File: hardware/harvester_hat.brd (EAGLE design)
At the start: 65 x 56.5 mm, 11 parts, among them IC1 7805T, J1 DCJ0202, U1 CAT24C32

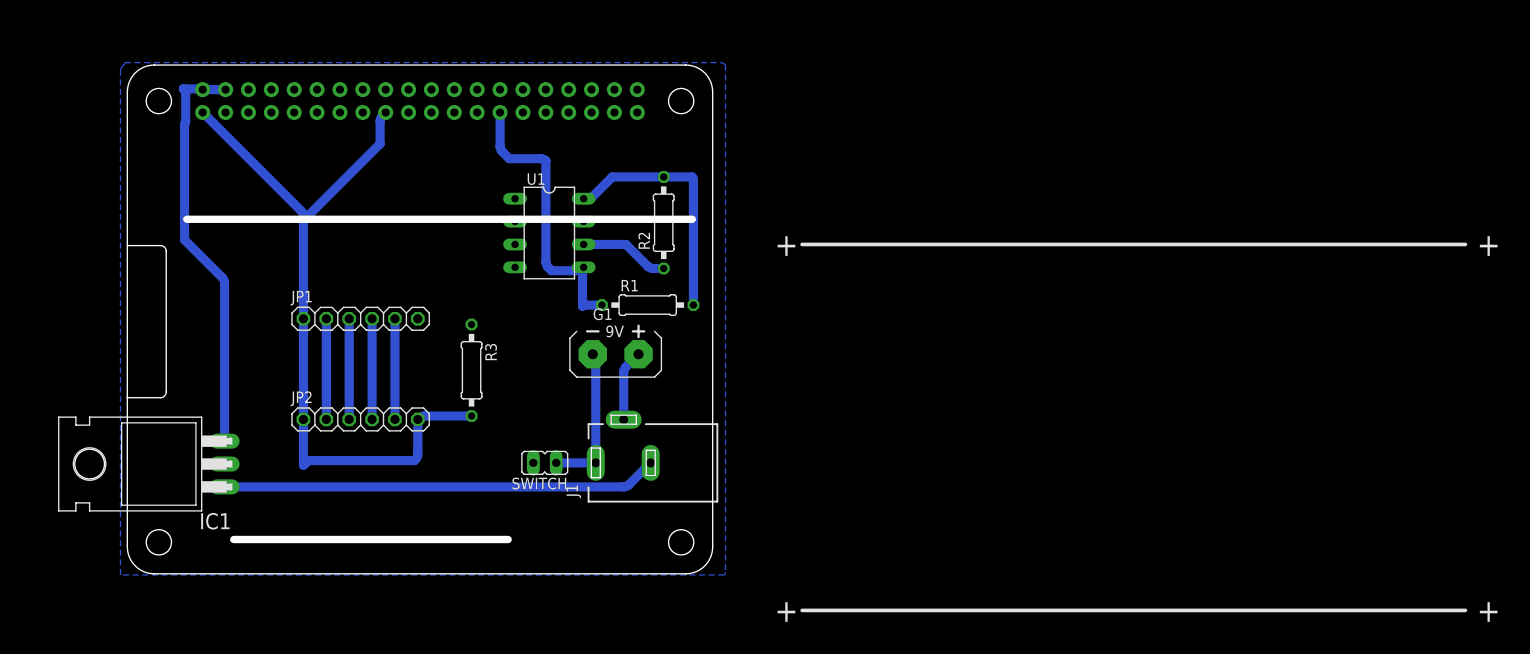
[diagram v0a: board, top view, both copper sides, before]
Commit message: added extra files
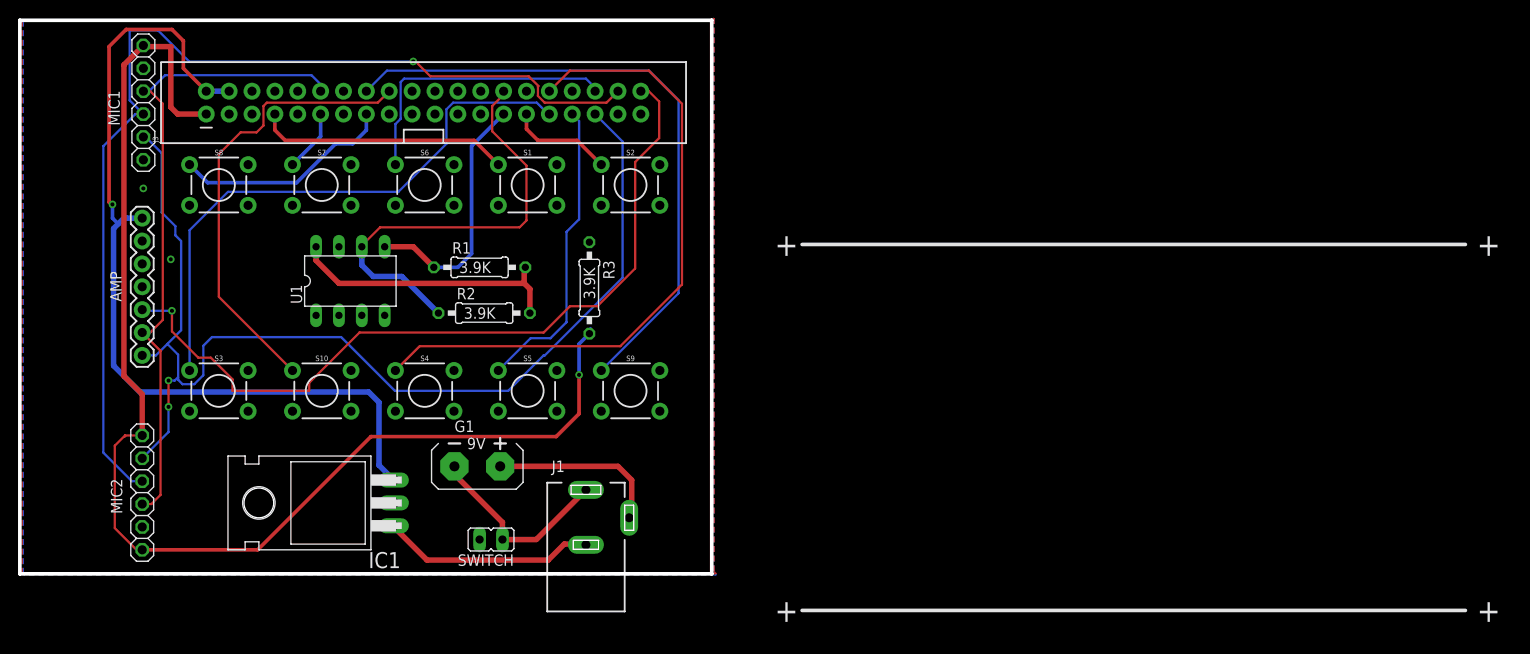
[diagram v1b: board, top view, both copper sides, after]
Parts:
- removed JP1, JP2: (no value), adafruit:1X06
- removed RPI1: RASPBERRYPI_BPLUS_HATNOSLOTS, microbuilder:PI_HAT_NOSLOTS
- added AMP: (no value), SparkFun-Connectors:1X07
- added J3: RASPBERRYPI-40-PIN-GPIO_PTH, SparkFun-Connectors:2X20_SHROUDED
- added MIC1, MIC2: (no value), adafruit:1X06
- added S1, S10, S2, S3, S4, S5, S6, S7, S8, S9: MOMENTARY-SWITCH-SPST-PTH-6.0MM, SparkFun-Switches:TACTILE_SWITCH_PTH_6.0MM
- moved U1 22.7 mm to (24.8, 32.5), turned to 0 degrees
- moved R2 22.3 mm to (39.6, 29.0), turned to 0 degrees
- moved G1 19.8 mm to (38.9, 11.9)
- moved IC1 19.3 mm to (19.4, 7.87)
- moved R1 19.1 mm to (39.1, 34.0)
- moved R3 16.0 mm to (51.3, 31.8)
- moved SWITCH 10.4 mm to (40.4, 3.81)
- moved J1 7.40 mm to (50.9, 6.22), turned to 0 degrees
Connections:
- new net N$7: AMP.5
- new net N$8: AMP.4
- net 3.3V: now also J3.1, J3.17, MIC1.1, MIC2.1, MIC2.6; no longer JP1.1, JP2.1, JP2.6, RPI1.1, RPI1.17
- net 5.0V: now also AMP.7, J3.2, J3.4; no longer RPI1.2, RPI1.4
- net EECLK: now also J3.28; no longer RPI1.28
- net EEDATA: now also J3.27; no longer RPI1.27
- net GND: now also AMP.6, J3.14, J3.20, J3.25, J3.30, J3.34, J3.39, J3.6, J3.9, MIC1.2, MIC1.6, MIC2.2, S1.3, S10.3, S2.3, S3.3, S4.3, S5.3, S6.3, S7.3, S8.3, S9.3; no longer JP1.2, JP1.6, JP2.2, RPI1.14, RPI1.20, RPI1.25, RPI1.30, RPI1.34, RPI1.39, RPI1.6, RPI1.9
- net GPIO12: now also J3.32, S4.1; no longer RPI1.32
- net GPIO13: now also J3.33, S5.1; no longer RPI1.33
- net GPIO16: now also J3.36, S6.1; no longer RPI1.36
- net GPIO17: now also J3.11, S7.1; no longer RPI1.11
- net GPIO18: now also AMP.2, J3.12, MIC1.3, MIC2.3; no longer JP1.3, JP2.3, RPI1.12
- net GPIO19: now also AMP.1, J3.35, MIC1.5, MIC2.5; no longer JP1.5, JP2.5, RPI1.35
- net GPIO20: now also J3.38, MIC1.4, MIC2.4; no longer JP1.4, JP2.4, RPI1.38
- net GPIO21: now also AMP.3, J3.40; no longer RPI1.40
- net GPIO22: now also J3.15, S8.1; no longer RPI1.15
- net GPIO23: now also J3.16, S9.1; no longer RPI1.16
- net GPIO24: now also J3.18, S10.1; no longer RPI1.18
- net GPIO25: now also J3.22; no longer RPI1.22
- net GPIO26: now also J3.37; no longer RPI1.37
- net GPIO27: now also J3.13; no longer RPI1.13
- net GPIO4: now also J3.7, S1.1; no longer RPI1.7
- net GPIO5: now also J3.29, S2.1; no longer RPI1.29
- net GPIO6: now also J3.31, S3.1; no longer RPI1.31
- net RXD: now also J3.10; no longer RPI1.10
- net SCL: now also J3.5; no longer RPI1.5
- net SDA: now also J3.3; no longer RPI1.3
- net SPI_CE0: now also J3.24; no longer RPI1.24
- net SPI_CE1: now also J3.26; no longer RPI1.26
- net SPI_MISO: now also J3.21; no longer RPI1.21
- net SPI_MOSI: now also J3.19; no longer RPI1.19
- net SPI_SCLK: now also J3.23; no longer RPI1.23
- net TXD: now also J3.8; no longer RPI1.8
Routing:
- net GPIO19: track 11.2 -> 126.4 mm, vias 0 -> 2
- net GPIO20: track 11.2 -> 116.2 mm, vias 0 -> 1
- net GPIO21: track 0.00 -> 88.9 mm, vias 0 -> 1
- net GPIO12: track 0.00 -> 73.1 mm
- net GPIO23: track 0.00 -> 70.5 mm
- net GPIO6: track 0.00 -> 64.2 mm
- net GPIO18: track 11.2 -> 72.5 mm
- net 3.3V: track 83.0 -> 140.8 mm, vias 0 -> 1
- net 5.0V: track 45.7 -> 99.2 mm, vias 0 -> 1
- net GPIO24: track 0.00 -> 50.5 mm
- net EECLK: track 9.94 -> 48.8 mm
- net GPIO13: track 0.00 -> 35.0 mm
- net GPIO16: track 0.00 -> 32.0 mm
- net GPIO4: track 0.00 -> 28.2 mm
- net GPIO22: track 0.00 -> 24.7 mm
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- added copper zone on layer 1, net GND
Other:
- board size 65 x 56.5 mm -> 76.8 x 61.5 mm
